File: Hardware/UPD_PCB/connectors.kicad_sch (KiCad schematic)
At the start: 27 parts, among them J1 25A Fuse holder, J10 796739-2, J11 Conn_01x02, J12 Conn_01x01, J2 796739-2, J3 Conn_01x02, J4 1776119-2, J5 1776119-2, J6 1776119-2, J7 1776119-2, J8 1776119-2, J9 1776119-2

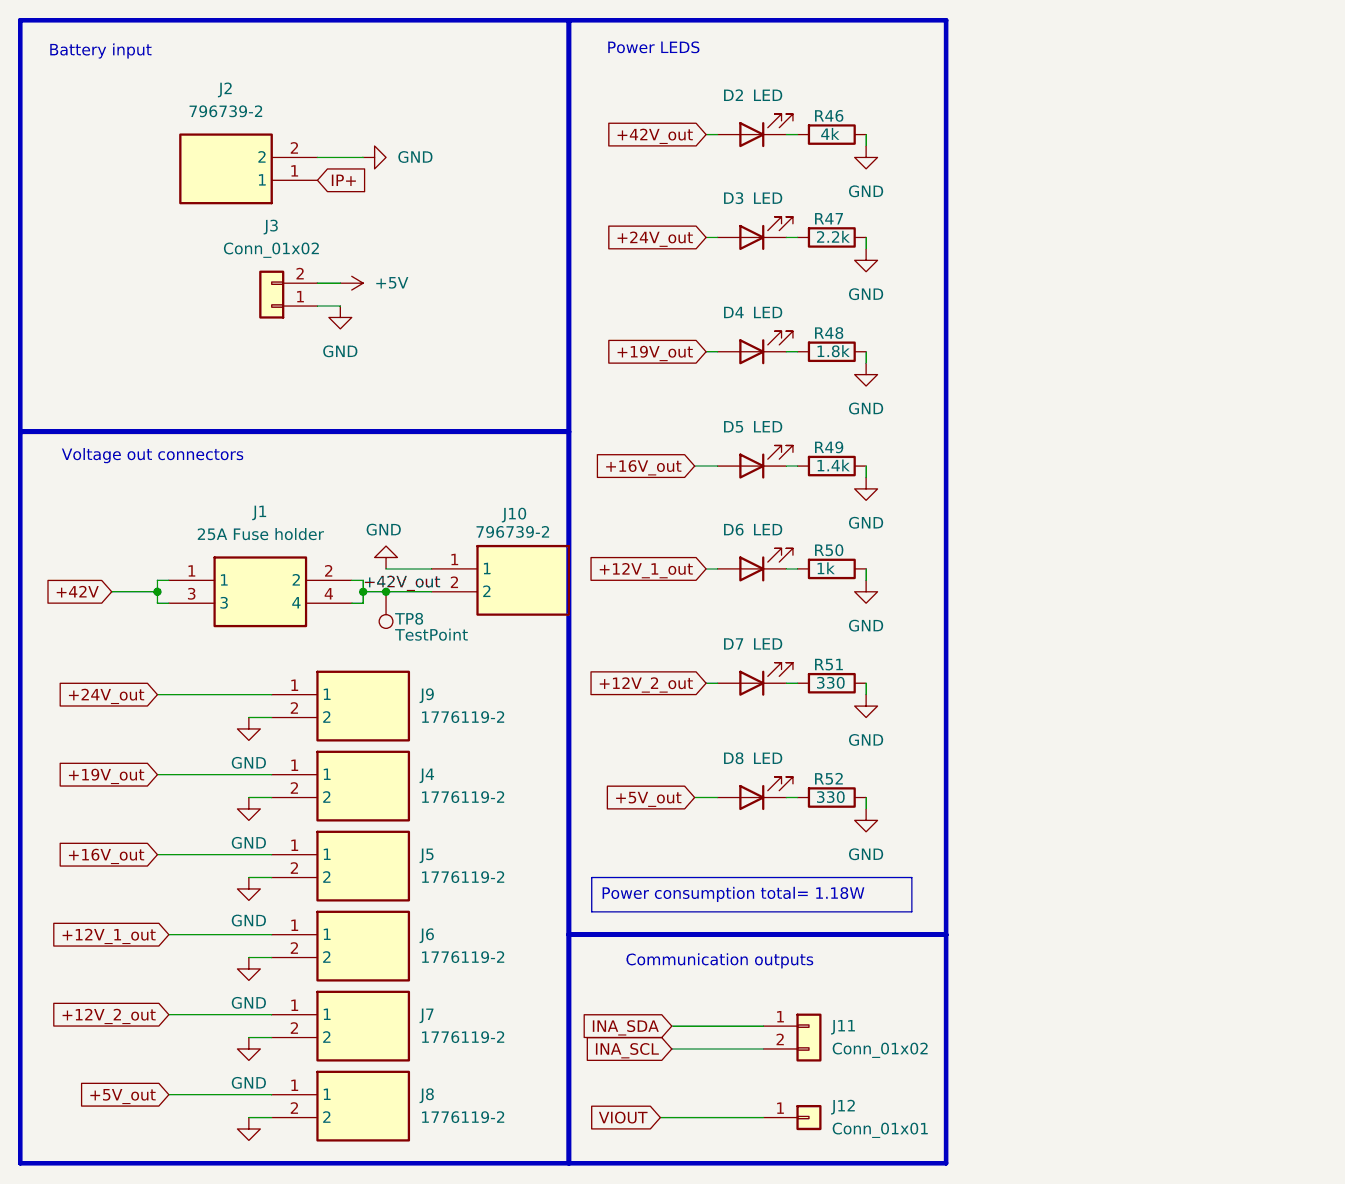
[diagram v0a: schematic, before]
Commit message: Finalized PCB
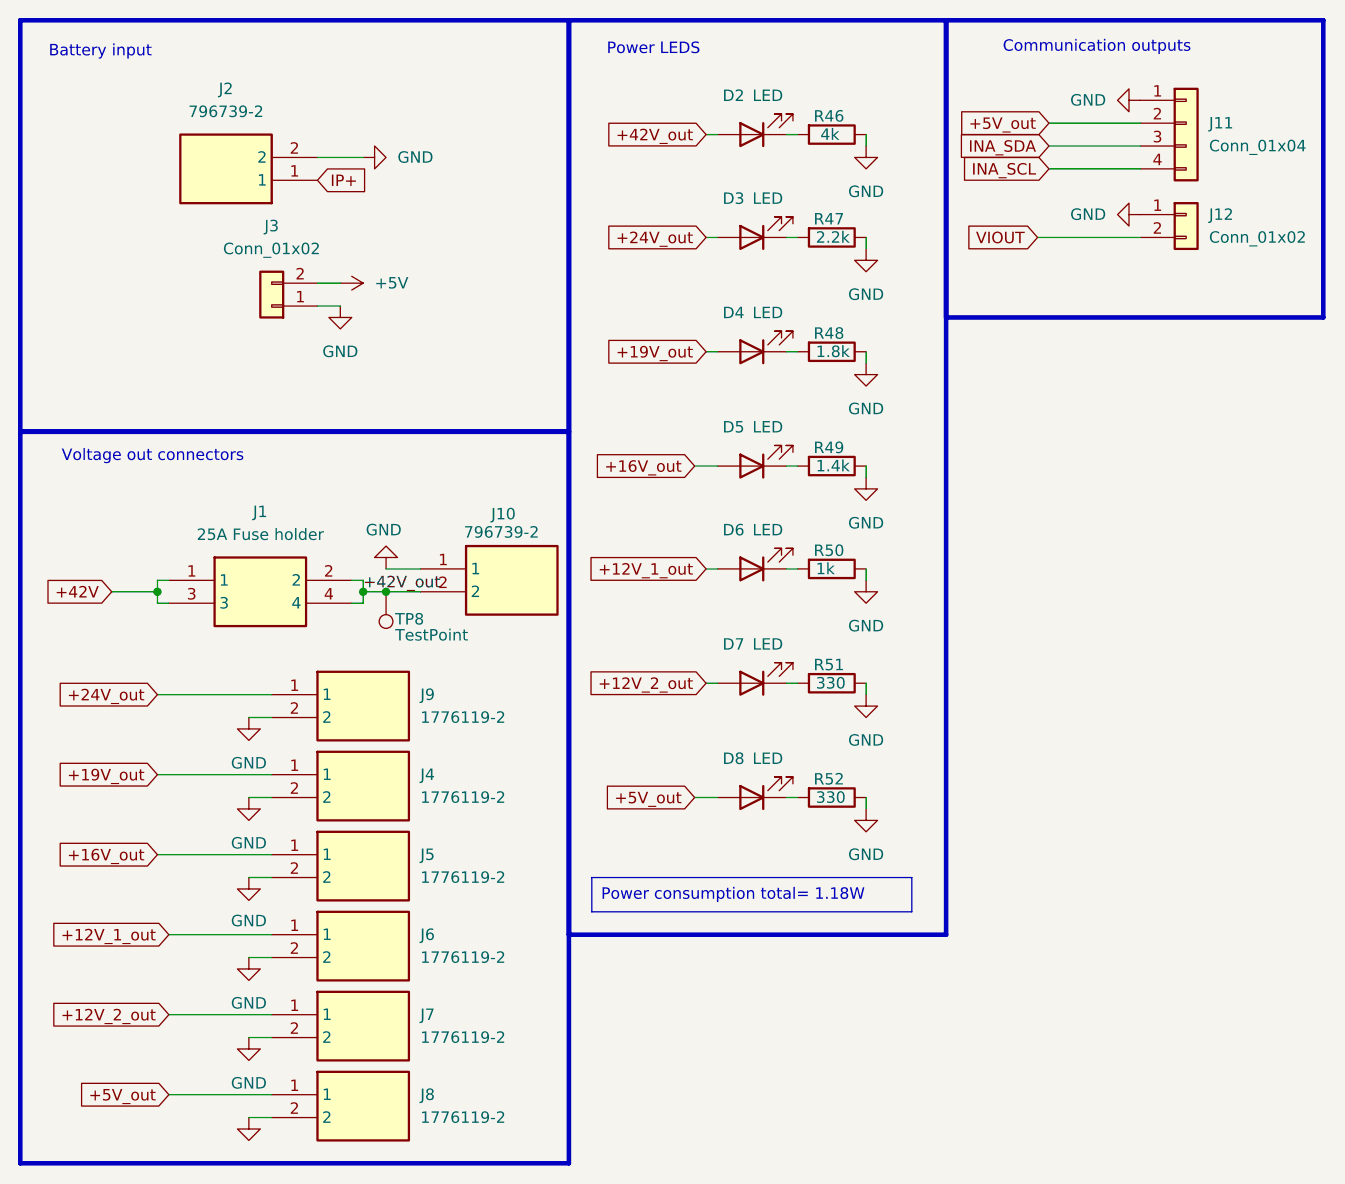
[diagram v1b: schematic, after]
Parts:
- removed J11: Conn_01x02, Connector_PinHeader_1.00mm:PinHeader_1x02_P1.00mm_Vertical, symbol Connector_Generic:Conn_01x02
- removed J12: Conn_01x01, Connector_PinHeader_1.00mm:PinHeader_1x01_P1.00mm_Vertical, symbol Connector_Generic:Conn_01x01
- added J11: Conn_01x04, Connector:NS-Tech_Grove_1x04_P2mm_Vertical, symbol Connector_Generic:Conn_01x04
- added J12: Conn_01x02, Connector_PinHeader_1.00mm:PinHeader_1x02_P1.00mm_Vertical, symbol Connector_Generic:Conn_01x02
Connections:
- net +5V_out: now also J11.2 (Pin_2)
- net GND: now also J11.1 (Pin_1), J12.1 (Pin_1)
- net INA_SCL: now also J11.4 (Pin_4)
- net INA_SDA: now also J11.3 (Pin_3)
- net VIOUT: now also J12.2 (Pin_2)
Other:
- moved on the sheet: J10
